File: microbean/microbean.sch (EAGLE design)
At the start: 18 parts, among them IC1 L78L33/L78L05, IC2 ST485/ST3485, IC3 PIC16F1827SO

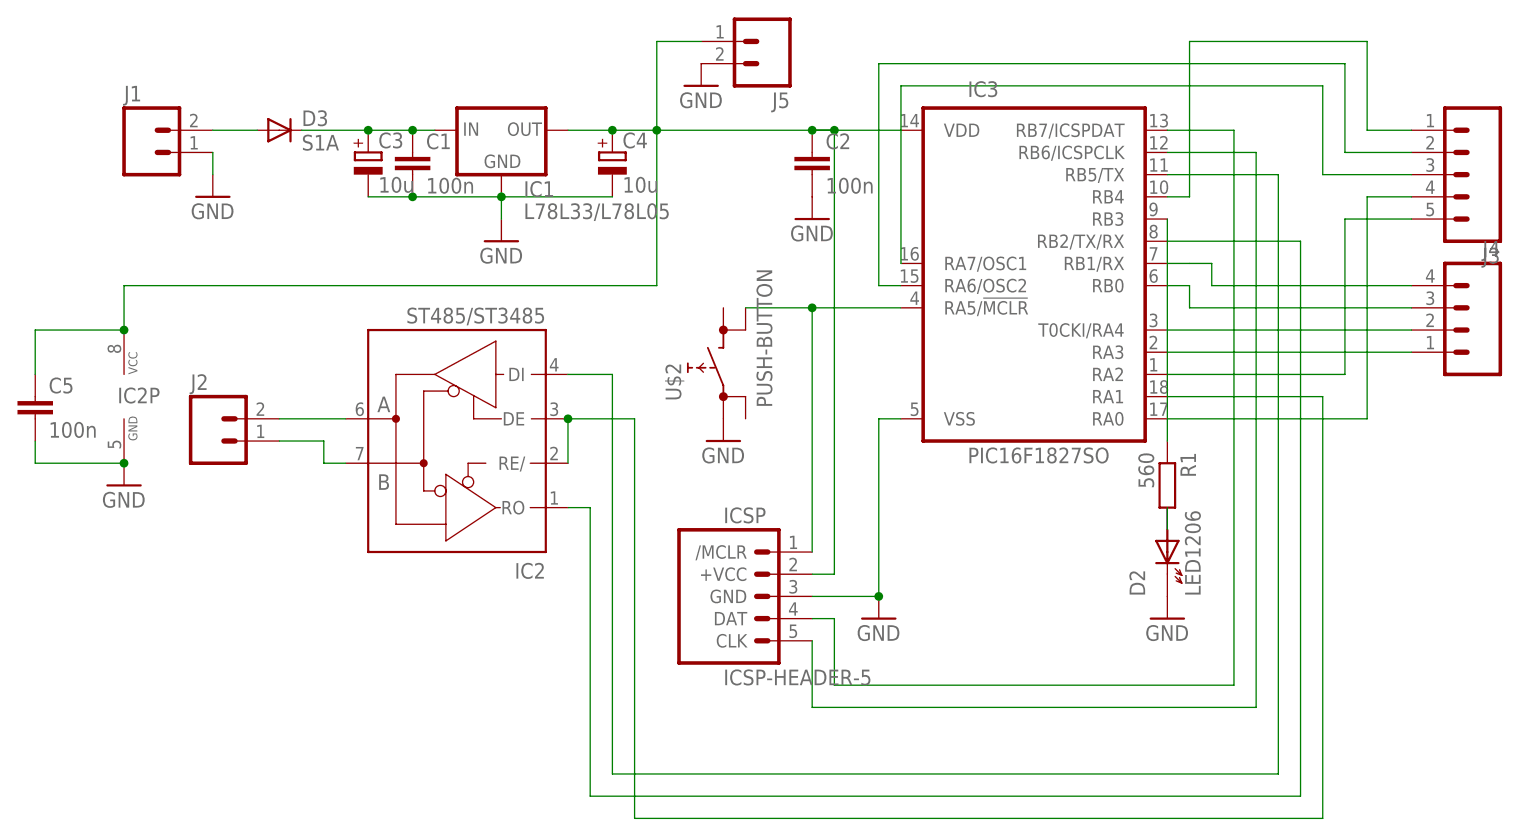
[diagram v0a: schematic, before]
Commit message: - Finishing up for quoting
git-svn-id: svn://mule/net/hardware/trunk@564 1a6b750e-079f-425f-90e7-3a118970be6b
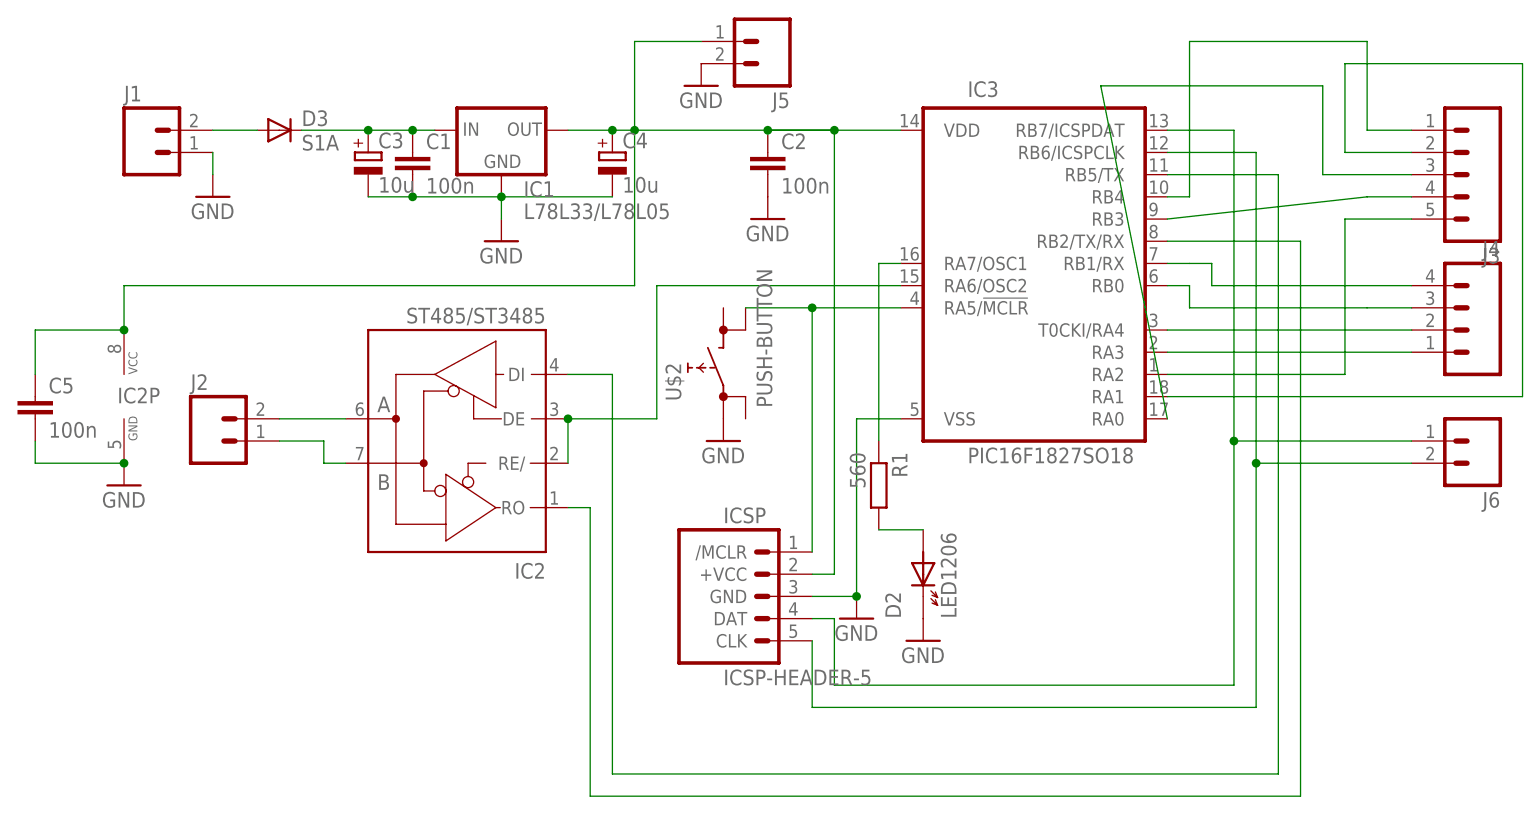
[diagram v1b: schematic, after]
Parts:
- added J6: (no value), custom:M02
- IC3: value PIC16F1827SO -> PIC16F1827SO18; device custom:PIC16F1827SO -> custom:PIC16F1827SO18
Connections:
- net N$11 renamed RB5
- net N$12 renamed RB2
- removed net CLK: IC3.RB6/ICSPCLK, ICSP.CLK
- removed net DAT: IC3.RB7/ICSPDAT, ICSP.DAT
- removed net RA6: IC3.RA6/OSC2, J3.2
- removed net RA7: IC3.RA7/OSC1, J3.3
- new net RA1: IC3.RA1, J3.2
- new net RB3: IC3.RB3, J3.4
- new net RB6: IC3.RB6/ICSPCLK, ICSP.CLK, J6.2
- new net RB7: IC3.RB7/ICSPDAT, ICSP.DAT, J6.1
- net N$23: now also IC3.RA6/OSC2; no longer IC3.RA1
- net N$9: now also IC3.RA7/OSC1; no longer IC3.RB3
- net RA0: now also J3.3; no longer J3.4
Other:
- moved on the sheet: C2, D2, R1

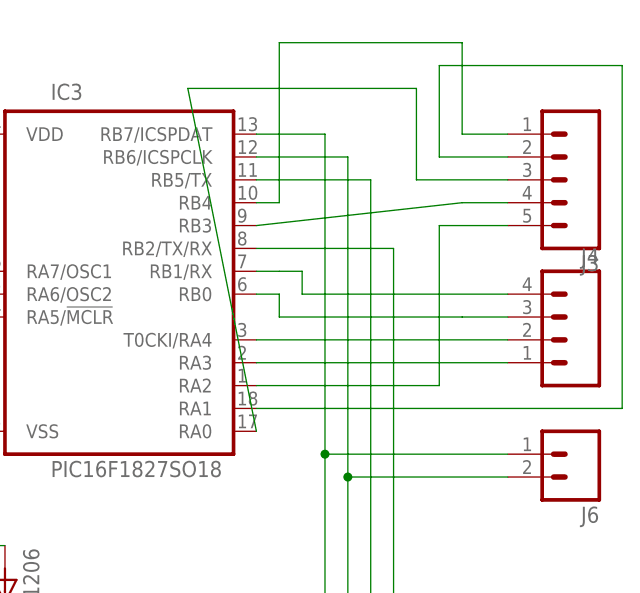
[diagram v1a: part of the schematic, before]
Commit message: - Ready for printing, optimized
git-svn-id: svn://mule/net/hardware/trunk@565 1a6b750e-079f-425f-90e7-3a118970be6b
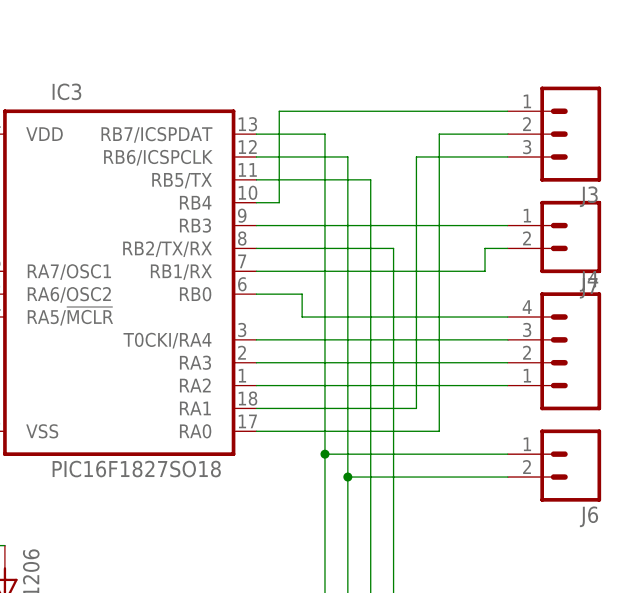
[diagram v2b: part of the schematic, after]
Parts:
- added J7: (no value), custom:M02
- J3: device custom:M05PTH -> custom:M03
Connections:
- net N$23 renamed RA6
- net N$9 renamed RA7
- net RA0: now also J3.2; no longer J3.3
- net RA1: now also J3.3; no longer J3.2
- net RA2: now also J4.1; no longer J3.5
- net RA3: now also J4.2; no longer J4.1
- net RA4: now also J4.3; no longer J4.2
- net RB0: now also J4.4; no longer J4.3
- net RB1: now also J7.2; no longer J4.4
- net RB3: now also J7.1; no longer J3.4
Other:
- moved on the sheet: J4
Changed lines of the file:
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@@
 <class number="0" name="default" width="0" drill="0">
+</class>
+<class number="1" name="power" width="0.508" drill="0">
 </class>
 </classes>
@@
 <part name="GND7" library="custom" deviceset="GND" device=""/>
 <part name="C5" library="custom" deviceset="C-EU" device="C0805" value="100n"/>
-<part name="J3" library="custom" deviceset="M05" device="PTH"/>
+<part name="J3" library="custom" deviceset="M03" device=""/>
 <part name="J4" library="custom" deviceset="M04" device=""/>
 <part name="J5" library="custom" deviceset="M02" device=""/>
 <part name="GND8" library="custom" deviceset="GND" device=""/>
 <part name="J6" library="custom" deviceset="M02" device=""/>
+<part name="J7" library="custom" deviceset="M02" device=""/>
 </parts>
 <sheets>
@@
 <instance part="GND7" gate="1" x="-17.78" y="33.02"/>
 <instance part="C5" gate="G$1" x="-27.94" y="43.18"/>
-<instance part="J3" gate="G$1" x="137.16" y="68.58" rot="R180"/>
-<instance part="J4" gate="G$1" x="137.16" y="53.34" rot="MR0"/>
+<instance part="J3" gate="G$1" x="137.16" y="73.66" rot="R180"/>
+<instance part="J4" gate="G$1" x="137.16" y="50.8" rot="MR0"/>
 <instance part="J5" gate="G$1" x="55.88" y="83.82" rot="R180"/>
 <instance part="GND8" gate="1" x="48.26" y="78.74"/>
 <instance part="J6" gate="G$1" x="137.16" y="38.1" rot="R180"/>
+<instance part="J7" gate="G$1" x="137.16" y="63.5" rot="R180"/>
 </instances>
 <busses>
@@
 <pinref part="GND1" gate="1" pin="GND"/>
 <pinref part="J1" gate="G$1" pin="1"/>
-<wire x1="-7.62" y1="68.58" x2="-7.62" y2="71.12" width="0.1524" layer="91"/>
+<wire x1="-7.62" y1="68.58" x2="-7.62" y2="71.12" width="0.508" layer="91"/>
 </segment>
 <segment>
 <pinref part="GND2" gate="1" pin="GND"/>
 <pinref part="IC1" gate="1" pin="GND"/>
-<wire x1="25.4" y1="63.5" x2="25.4" y2="66.04" width="0.1524" layer="91"/>
+<wire x1="25.4" y1="63.5" x2="25.4" y2="66.04" width="0.508" layer="91"/>
 <pinref part="C3" gate="G$1" pin="-"/>
 <pinref part="C1" gate="G$1" pin="2"/>
@@
 </segment>
 </net>
-<net name="N$1" class="0">
+<net name="N$1" class="1">
 <segment>
 <pinref part="J1" gate="G$1" pin="2"/>
@@
 </segment>
 </net>
-<net name="N$2" class="0">
+<net name="N$2" class="1">
 <segment>
 <pinref part="IC1" gate="1" pin="IN"/>
 <pinref part="D3" gate="G$1" pin="C"/>
-<wire x1="2.54" y1="73.66" x2="10.16" y2="73.66" width="0.1524" layer="91"/>
+<wire x1="2.54" y1="73.66" x2="10.16" y2="73.66" width="0.508" layer="91"/>
 <pinref part="C1" gate="G$1" pin="1"/>
-<wire x1="10.16" y1="73.66" x2="15.24" y2="73.66" width="0.1524" layer="91"/>
-<wire x1="15.24" y1="73.66" x2="17.78" y2="73.66" width="0.1524" layer="91"/>
+<wire x1="10.16" y1="73.66" x2="15.24" y2="73.66" width="0.508" layer="91"/>
+<wire x1="15.24" y1="73.66" x2="17.78" y2="73.66" width="0.508" layer="91"/>
 <junction x="15.24" y="73.66"/>
 <pinref part="C3" gate="G$1" pin="+"/>
@@
 </segment>
 </net>
-<net name="N$9" class="0">
+<net name="RA7" class="0">
 <segment>
 <pinref part="IC3" gate="G$1" pin="RA7/OSC1"/>
@@
 </segment>
 </net>
-<net name="RB1" class="0">
-<segment>
-<pinref part="IC3" gate="G$1" pin="RB1/RX"/>
+<net name="RB0" class="0">
+<segment>
+<pinref part="IC3" gate="G$1" pin="RB0"/>
 <pinref part="J4" gate="G$1" pin="4"/>
-<wire x1="101.6" y1="58.42" x2="104.14" y2="58.42" width="0.1524" layer="91"/>
-<wire x1="129.54" y1="55.88" x2="106.68" y2="55.88" width="0.1524" layer="91"/>
-<wire x1="106.68" y1="55.88" x2="106.68" y2="58.42" width="0.1524" layer="91"/>
-<wire x1="106.68" y1="58.42" x2="104.14" y2="58.42" width="0.1524" layer="91"/>
-</segment>
-</net>
-<net name="RB0" class="0">
-<segment>
-<pinref part="IC3" gate="G$1" pin="RB0"/>
-<wire x1="101.6" y1="55.88" x2="104.14" y2="55.88" width="0.1524" layer="91"/>
-<wire x1="104.14" y1="55.88" x2="104.14" y2="53.34" width="0.1524" layer="91"/>
-<wire x1="104.14" y1="53.34" x2="124.46" y2="53.34" width="0.1524" layer="91"/>
+<wire x1="129.54" y1="53.34" x2="106.68" y2="53.34" width="0.1524" layer="91"/>
+<wire x1="106.68" y1="53.34" x2="106.68" y2="55.88" width="0.1524" layer="91"/>
+<wire x1="106.68" y1="55.88" x2="101.6" y2="55.88" width="0.1524" layer="91"/>
+</segment>
+</net>
+<net name="RA3" class="0">
+<segment>
+<pinref part="IC3" gate="G$1" pin="RA3"/>
+<wire x1="101.6" y1="48.26" x2="129.54" y2="48.26" width="0.1524" layer="91"/>
+<pinref part="J4" gate="G$1" pin="2"/>
+</segment>
+</net>
+<net name="RA4" class="0">
+<segment>
+<pinref part="IC3" gate="G$1" pin="T0CKI/RA4"/>
 <pinref part="J4" gate="G$1" pin="3"/>
-<wire x1="124.46" y1="53.34" x2="129.54" y2="53.34" width="0.1524" layer="91"/>
-</segment>
-</net>
-<net name="RA4" class="0">
-<segment>
-<pinref part="IC3" gate="G$1" pin="T0CKI/RA4"/>
-<pinref part="J4" gate="G$1" pin="2"/>
 <wire x1="101.6" y1="50.8" x2="129.54" y2="50.8" width="0.1524" layer="91"/>
 </segment>
 </net>
-<net name="RA3" class="0">
-<segment>
-<pinref part="IC3" gate="G$1" pin="RA3"/>
-<pinref part="J4" gate="G$1" pin="1"/>
-<wire x1="101.6" y1="48.26" x2="129.54" y2="48.26" width="0.1524" layer="91"/>
-</segment>
-</net>
-<net name="RA2" class="0">
-<segment>
-<pinref part="IC3" gate="G$1" pin="RA2"/>
-<wire x1="101.6" y1="45.72" x2="121.92" y2="45.72" width="0.1524" layer="91"/>
-<wire x1="121.92" y1="45.72" x2="121.92" y2="63.5" width="0.1524" layer="91"/>
-<wire x1="121.92" y1="63.5" x2="129.54" y2="63.5" width="0.1524" layer="91"/>
-<pinref part="J3" gate="G$1" pin="5"/>
-</segment>
-</net>
-<net name="RB3" class="0">
-<segment>
-<pinref part="IC3" gate="G$1" pin="RB3"/>
-<wire x1="101.6" y1="63.5" x2="124.46" y2="66.04" width="0.1524" layer="91"/>
-<pinref part="J3" gate="G$1" pin="4"/>
-<wire x1="124.46" y1="66.04" x2="129.54" y2="66.04" width="0.1524" layer="91"/>
-</segment>
-</net>
-<net name="RA0" class="0">
-<segment>
-<pinref part="IC3" gate="G$1" pin="RA0"/>
-<wire x1="101.6" y1="40.64" x2="93.98" y2="78.74" width="0.1524" layer="91"/>
-<wire x1="93.98" y1="78.74" x2="119.38" y2="78.74" width="0.1524" layer="91"/>
-<wire x1="119.38" y1="78.74" x2="119.38" y2="68.58" width="0.1524" layer="91"/>
+<net name="RA1" class="0">
+<segment>
+<pinref part="IC3" gate="G$1" pin="RA1"/>
+<wire x1="101.6" y1="43.18" x2="119.38" y2="43.18" width="0.1524" layer="91"/>
+<wire x1="119.38" y1="43.18" x2="119.38" y2="71.12" width="0.1524" layer="91"/>
 <pinref part="J3" gate="G$1" pin="3"/>
-<wire x1="119.38" y1="68.58" x2="129.54" y2="68.58" width="0.1524" layer="91"/>
+<wire x1="119.38" y1="71.12" x2="129.54" y2="71.12" width="0.1524" layer="91"/>
 </segment>
 </net>
@@
 <pinref part="IC3" gate="G$1" pin="RB4"/>
 <wire x1="101.6" y1="66.04" x2="104.14" y2="66.04" width="0.1524" layer="91"/>
-<wire x1="104.14" y1="66.04" x2="104.14" y2="83.82" width="0.1524" layer="91"/>
-<wire x1="104.14" y1="83.82" x2="124.46" y2="83.82" width="0.1524" layer="91"/>
-<wire x1="124.46" y1="83.82" x2="124.46" y2="73.66" width="0.1524" layer="91"/>
+<wire x1="104.14" y1="66.04" x2="104.14" y2="76.2" width="0.1524" layer="91"/>
+<wire x1="104.14" y1="76.2" x2="129.54" y2="76.2" width="0.1524" layer="91"/>
 <pinref part="J3" gate="G$1" pin="1"/>
-<wire x1="129.54" y1="73.66" x2="124.46" y2="73.66" width="0.1524" layer="91"/>
-</segment>
-</net>
-<net name="N$23" class="0">
+</segment>
+</net>
+<net name="RA6" class="0">
 <segment>
 <pinref part="IC3" gate="G$1" pin="RA6/OSC2"/>
@@
 </segment>
 </net>
-<net name="RA1" class="0">
-<segment>
-<pinref part="IC3" gate="G$1" pin="RA1"/>
-<wire x1="101.6" y1="43.18" x2="142.24" y2="43.18" width="0.1524" layer="91"/>
-<wire x1="142.24" y1="43.18" x2="142.24" y2="81.28" width="0.1524" layer="91"/>
-<wire x1="142.24" y1="81.28" x2="121.92" y2="81.28" width="0.1524" layer="91"/>
-<wire x1="121.92" y1="81.28" x2="121.92" y2="71.12" width="0.1524" layer="91"/>
+<net name="RA0" class="0">
+<segment>
+<pinref part="IC3" gate="G$1" pin="RA0"/>
+<wire x1="101.6" y1="40.64" x2="121.92" y2="40.64" width="0.1524" layer="91"/>
+<wire x1="121.92" y1="40.64" x2="121.92" y2="73.66" width="0.1524" layer="91"/>
 <pinref part="J3" gate="G$1" pin="2"/>
-<wire x1="121.92" y1="71.12" x2="129.54" y2="71.12" width="0.1524" layer="91"/>
-</segment>
-</net>
+<wire x1="121.92" y1="73.66" x2="129.54" y2="73.66" width="0.1524" layer="91"/>
+</segment>
+</net>
+<net name="RB3" class="0">
+<segment>
+<pinref part="IC3" gate="G$1" pin="RB3"/>
+<wire x1="101.6" y1="63.5" x2="129.54" y2="63.5" width="0.1524" layer="91"/>
+<pinref part="J7" gate="G$1" pin="1"/>
+</segment>
+</net>
+<net name="RA2" class="0">
+<segment>
+<pinref part="IC3" gate="G$1" pin="RA2"/>
+<pinref part="J4" gate="G$1" pin="1"/>
+<wire x1="101.6" y1="45.72" x2="129.54" y2="45.72" width="0.1524" layer="91"/>
+</segment>
+</net>
+<net name="RB1" class="0">
+<segment>
+<pinref part="IC3" gate="G$1" pin="RB1/RX"/>
+<wire x1="101.6" y1="58.42" x2="127" y2="58.42" width="0.1524" layer="91"/>
+<pinref part="J7" gate="G$1" pin="2"/>
+<wire x1="127" y1="58.42" x2="127" y2="60.96" width="0.1524" layer="91"/>
+<wire x1="127" y1="60.96" x2="129.54" y2="60.96" width="0.1524" layer="91"/>
+</segment>
+</net>
